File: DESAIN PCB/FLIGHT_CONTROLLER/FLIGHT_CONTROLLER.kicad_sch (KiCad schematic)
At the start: 49 parts, among them J1 POWER CONNECTOR, J10 ESC INPUT, J11 ESC INPUT, J12 RC TRANSMITTER, J13 TRANSMITTER, J14 GY-88A, J15 FTDI BREAKOUT BOARD, J16 ESC POWER, J2 SPI PROG, J3 USB B, J4 ESC INPUT, J5 ESC INPUT, J6 ESC POWER, J7 ESC POWER, J8 ESC POWER, J9 ESC POWER, SW1 SW_DPDT_x2, SW2 RESET BUTTON, U1 ATmega328P-A, U2 AMS1117-5.0, U3 FT232RL, Y1 16MHz

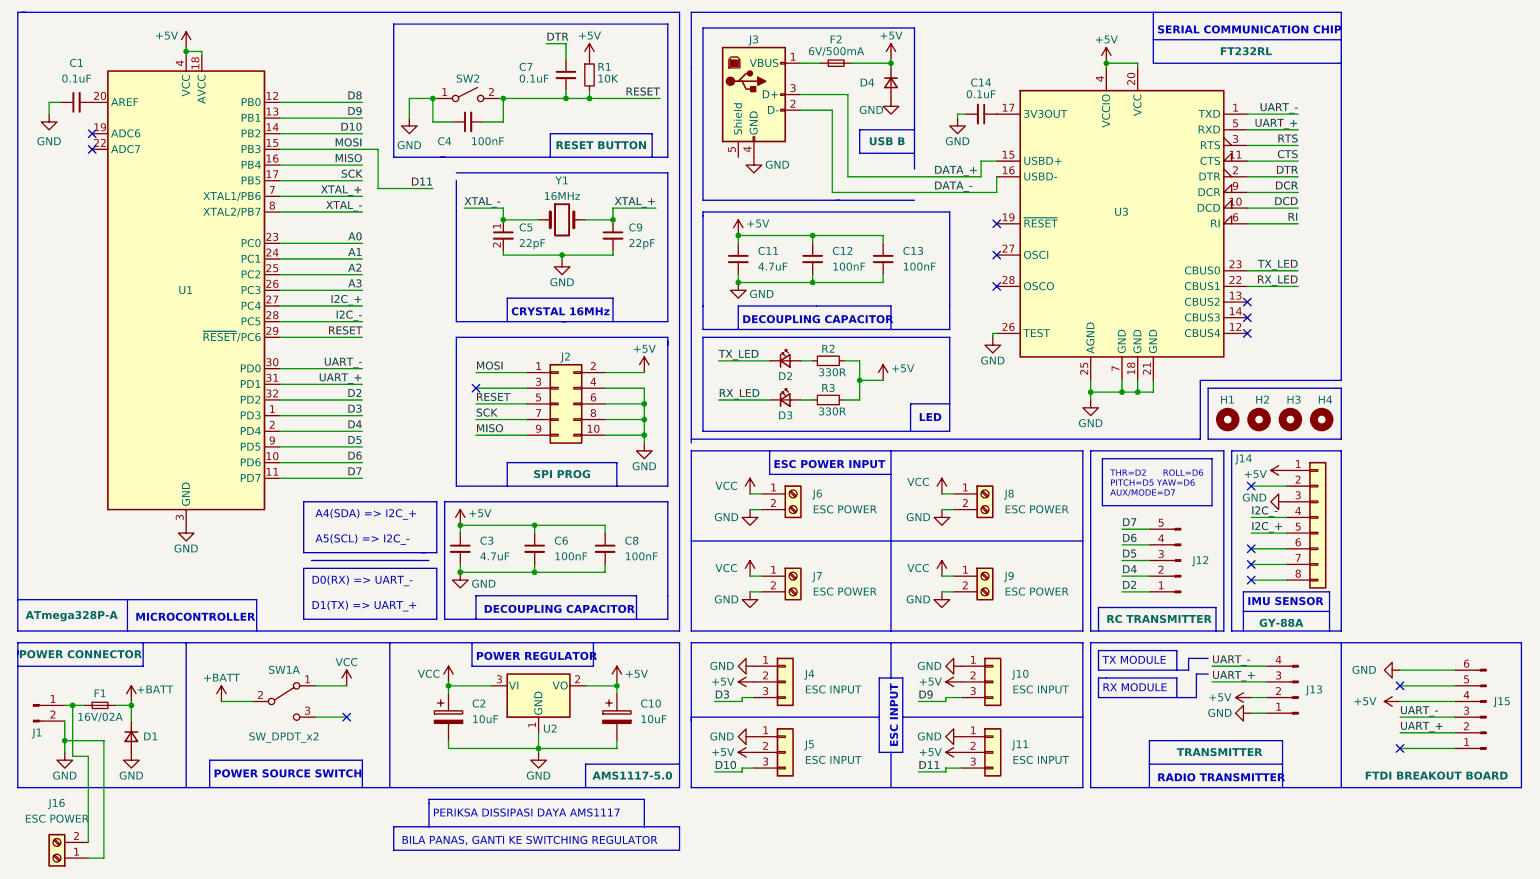
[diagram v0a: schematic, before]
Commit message: [Board] Review complete
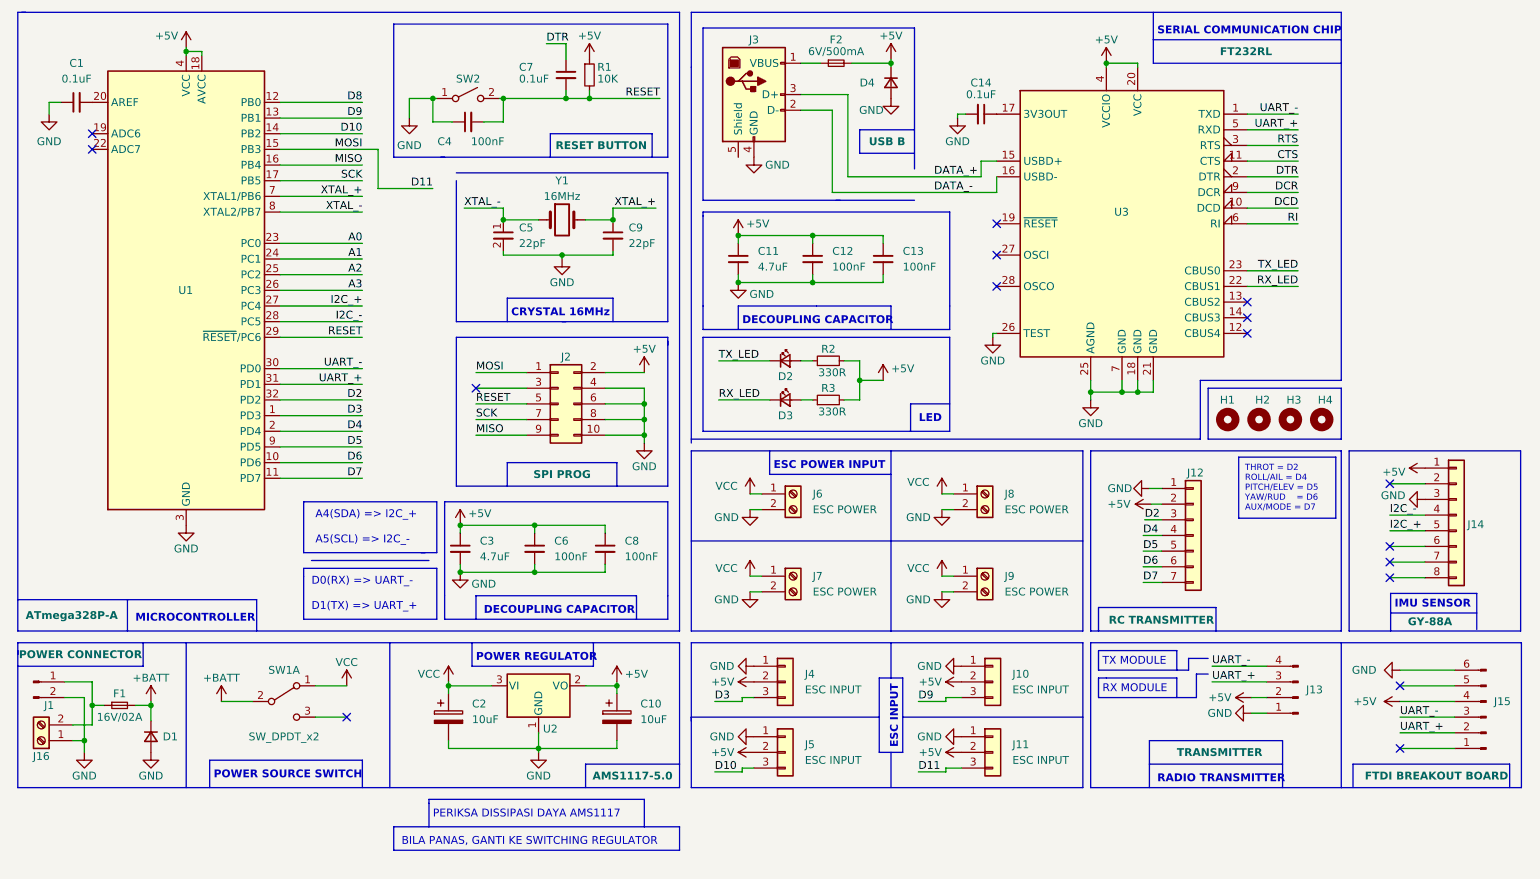
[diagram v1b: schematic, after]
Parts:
- removed J12: RC TRANSMITTER, Connector_PinSocket_2.54mm:PinSocket_1x05_P2.54mm_Vertical, symbol Connector:Conn_01x05_Male
- added J12: RC TRANSMITTER, Connector_PinSocket_2.54mm:PinSocket_1x07_P2.54mm_Vertical, symbol Connector_Generic:Conn_01x07
- J15: footprint Connector_PinHeader_2.54mm:PinHeader_1x06_P2.54mm_Vertical -> Connector_PinSocket_2.54mm:PinSocket_1x06_P2.54mm_Vertical
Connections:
- net +5V: now also J12.2 (Pin_2)
- net D2: now also J12.3 (Pin_3)
- net D4: now also J12.4 (Pin_4)
- net D5: now also J12.5 (Pin_5)
- net D6: now also J12.6 (Pin_6)
- net D7: now also J12.7 (Pin_7)
- net GND: now also J12.1 (Pin_1)
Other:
- note added: "THROT = D2 ROLL/AIL = D4 PITCH/ELEV = D5 YAW/RUD = D6 AUX/MODE = D7"
- note removed: "THR=D2 ROLL=D6 PITCH=D5 YAW=D6 AUX/MODE=D7"
- moved on the sheet: D1, F1, J1, J14, J16
